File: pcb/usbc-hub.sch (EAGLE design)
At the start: 88 parts, among them Q1 AO3401, Q2 AO3401, Q3 AO3401, Q4 AO3401, U1 HD3SS3220, U10 USB5826, U11 MIC24045, U2 MIC2019, U3 MIC2019, U4 MIC2019, U5 MIC2019, U6 UTC2000, U7 UTC2000, U8 MIC2019, U9 MIC2019, X1 25 MHz

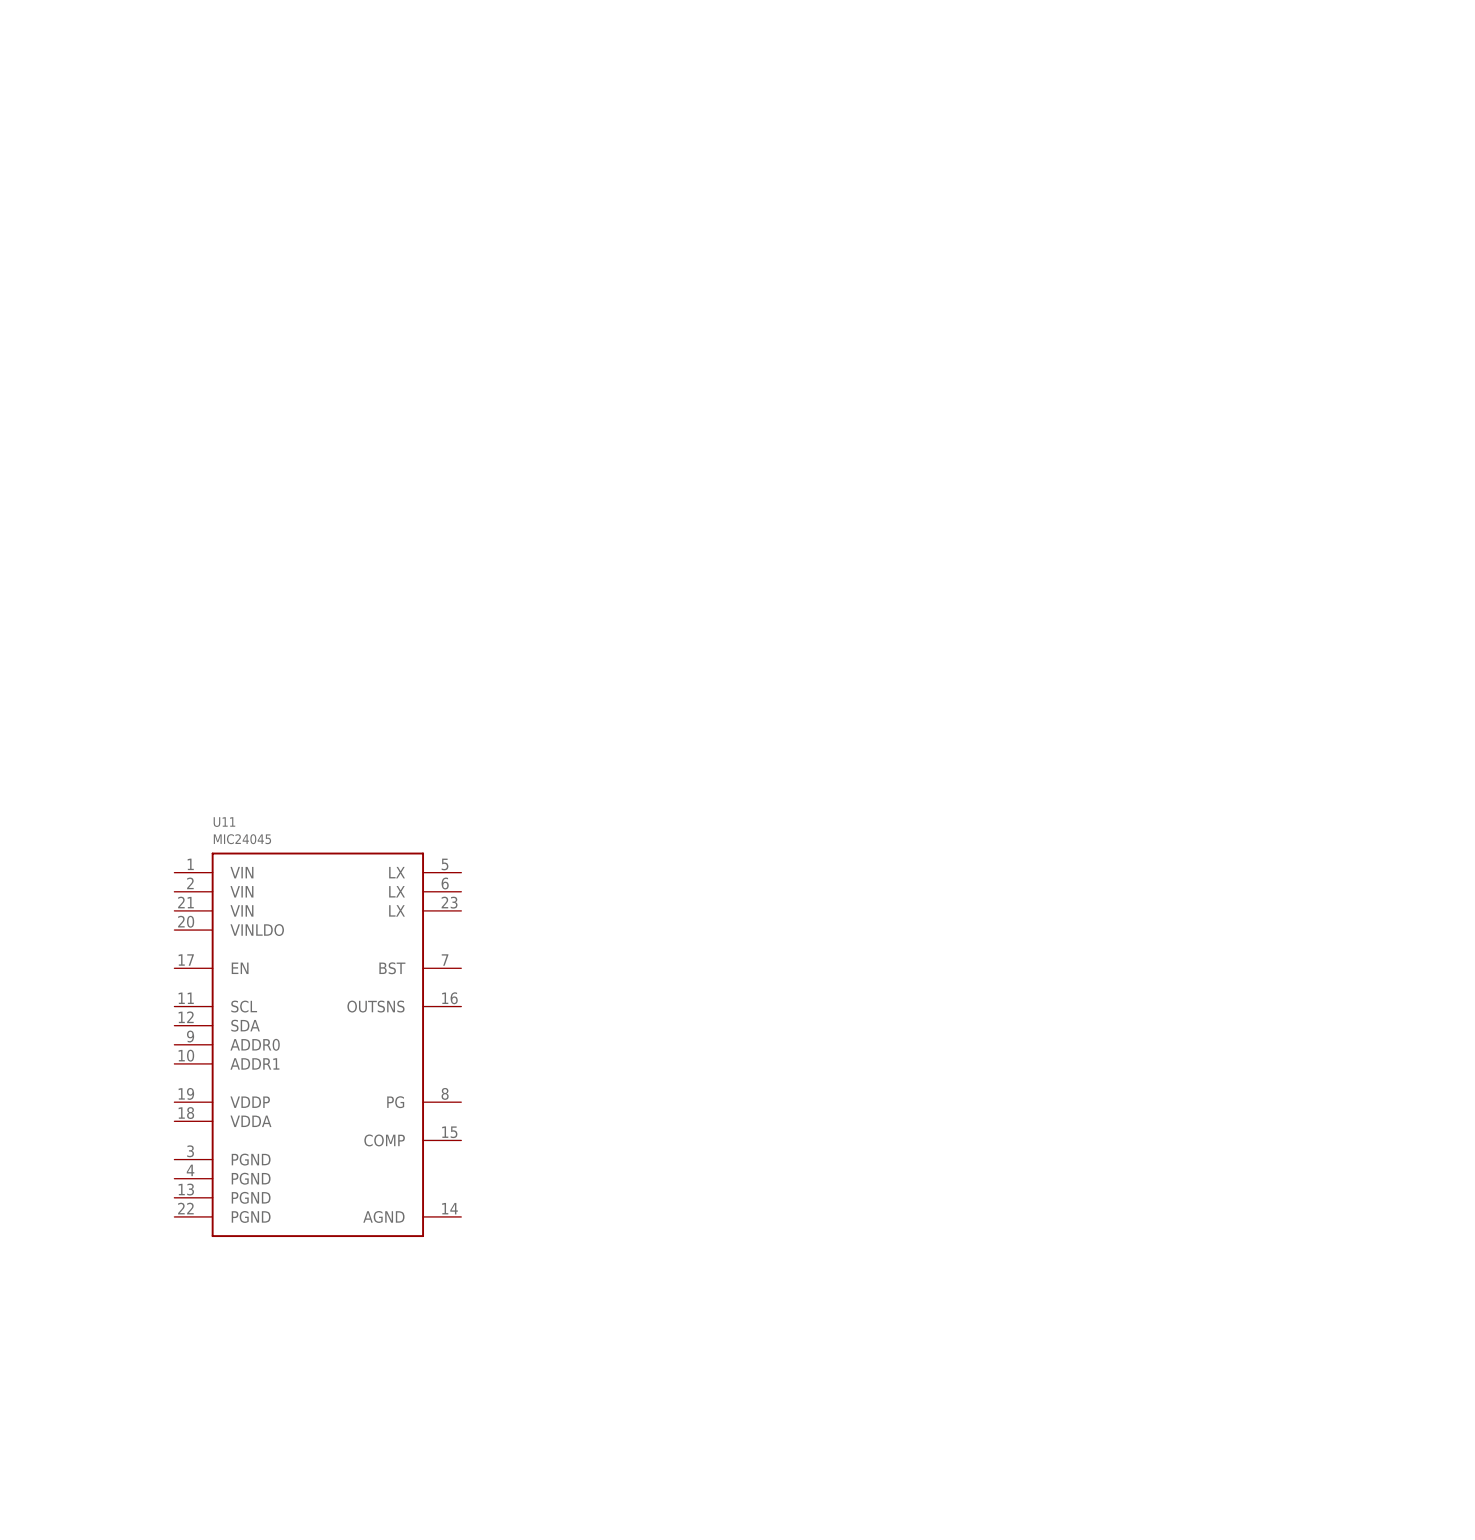
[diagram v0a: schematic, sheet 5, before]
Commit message: Work on power
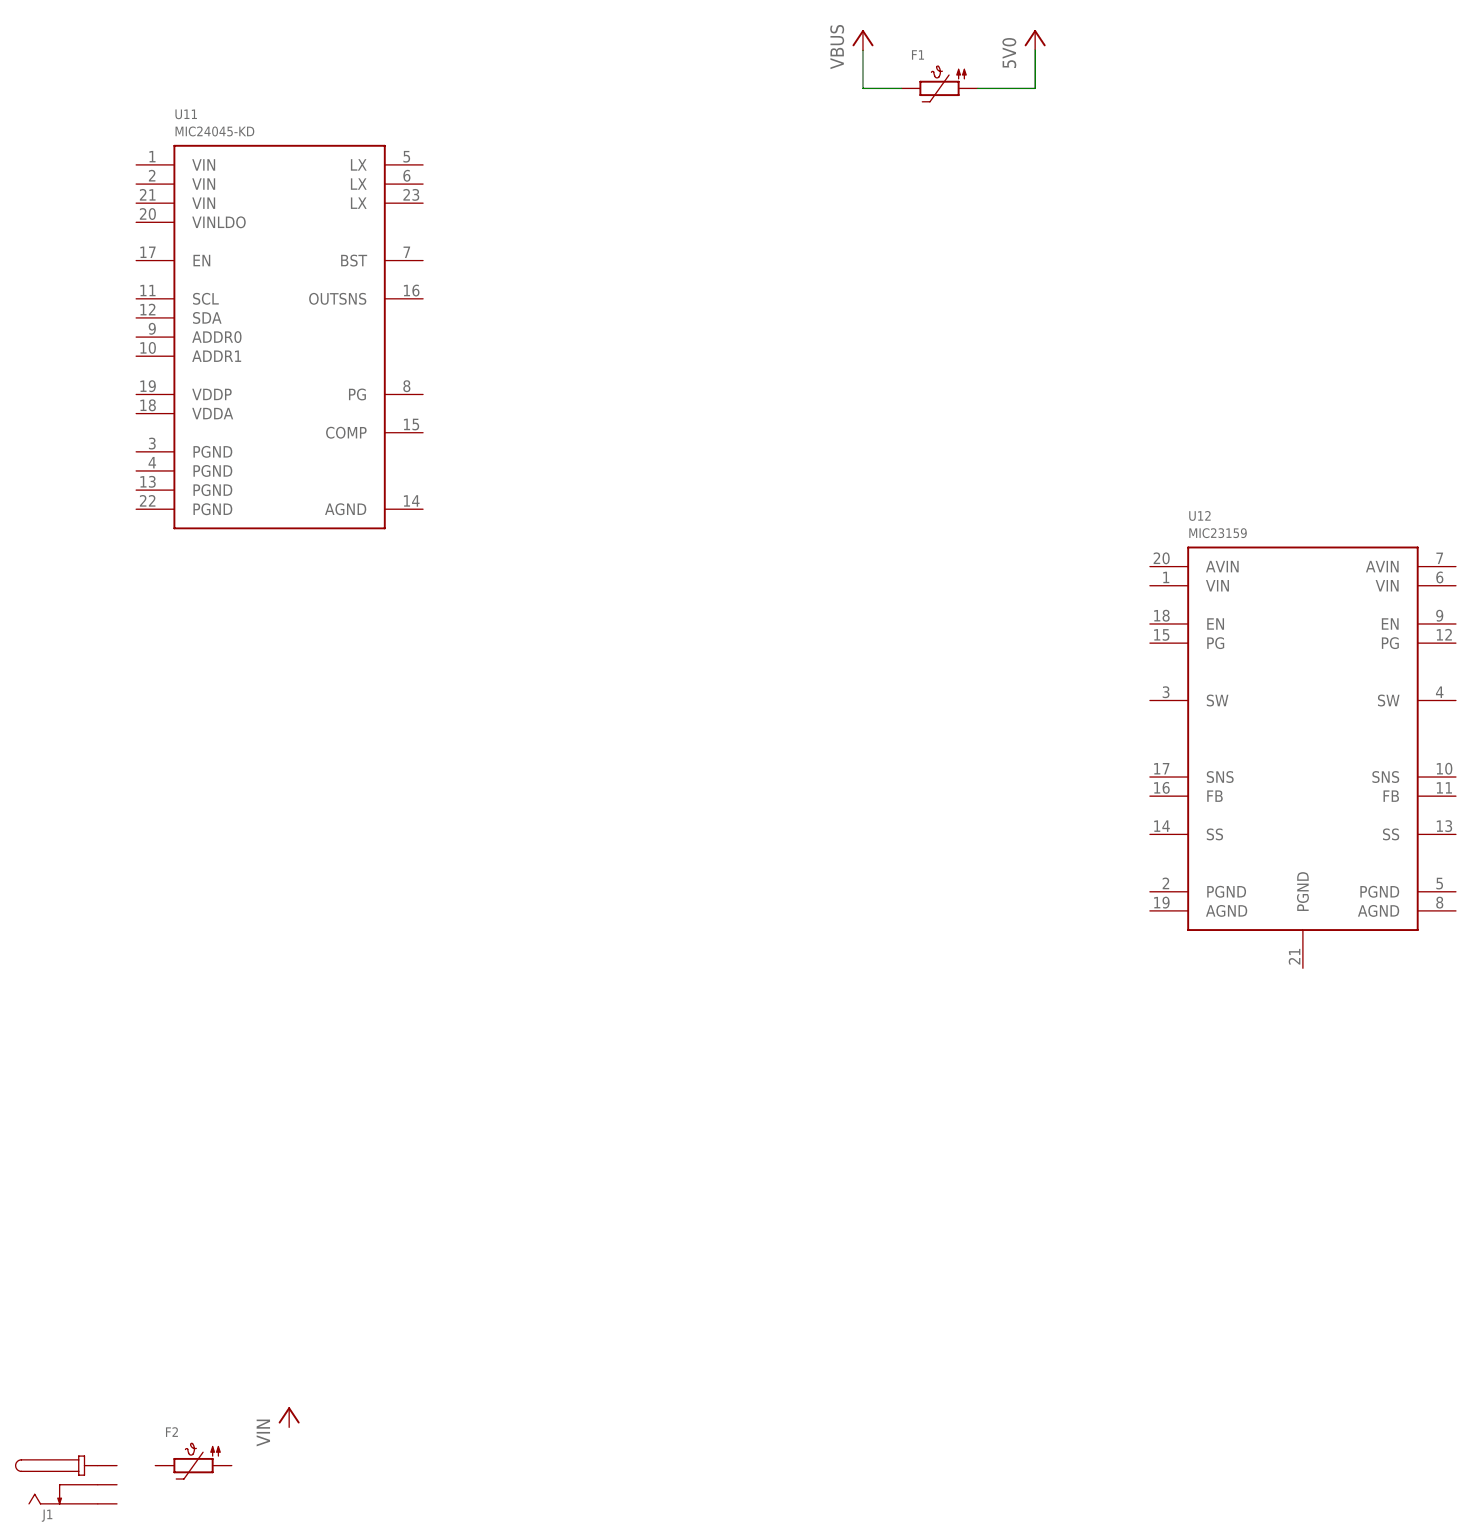
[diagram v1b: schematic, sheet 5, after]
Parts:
- added F1, F2: (no value), PTC Fuses:PTC1812
- added J1: DCJACK, DC Jack:DCJACK
- added R47, R48: 165 Ohms, Resistor:RESISTOR-0603
- added U12: MIC23159, Microchip:MIC23159
- U11: value MIC24045 -> MIC24045-KD; device Microchip:MIC24045 -> Microchip:MIC24045-KD
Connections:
- new net N$28: R47.1, U8.ILIMIT
- new net N$29: R48.1, U9.ILIMIT
- net 5V0: now also F1.1
- net GND: now also R47.2, R48.2, U8.GND, U9.GND
- net VBUS: now also F1.2
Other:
- moved on the sheet: U11
